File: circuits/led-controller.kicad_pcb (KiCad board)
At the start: 4 copper layers, 33.1 x 78.4 mm, 53 parts, among them J1 Conn_02x08_Odd_Even, Q1 Q_NPN_BEC, U1 ESP-WROOM-32, U2 IR-RX-TSOP34438, U3 SPH0645LM4H-B, U4 MCP73831T, U5 MAX98357AETE+T, U6 SI7020-A20, U7 PYQ2898, U7 housing-mounts, U8 TSL45315CL, U9 AP2112

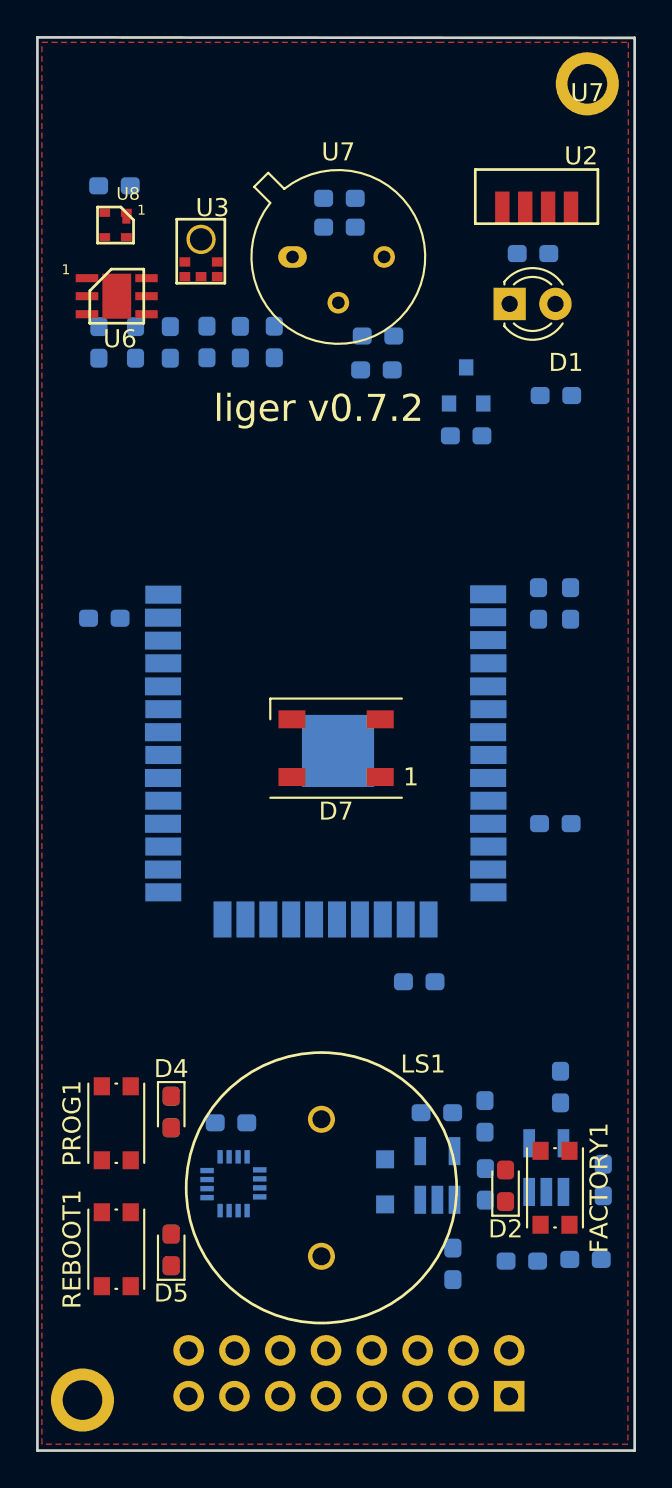
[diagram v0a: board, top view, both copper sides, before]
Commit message: sent to boardhouse
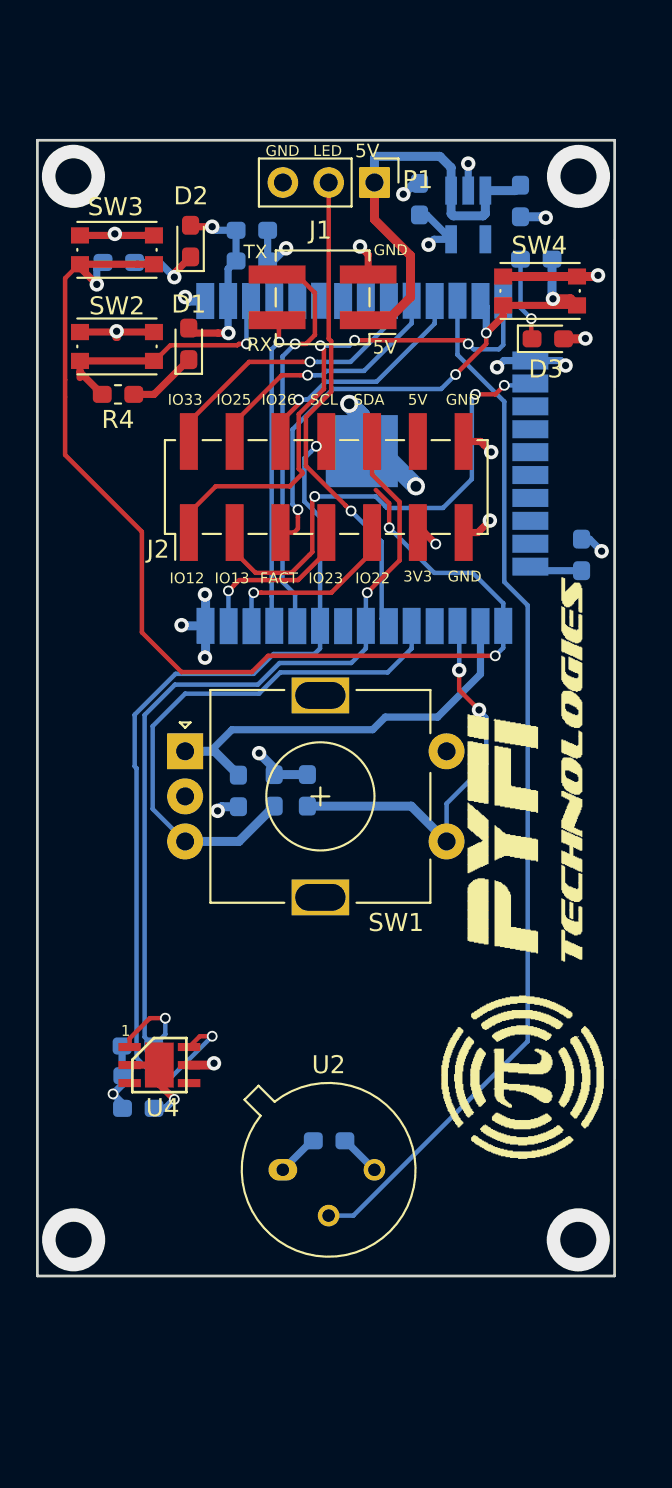
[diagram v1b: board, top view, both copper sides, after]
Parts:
- removed C10, C11: C_0.1uF, Capacitor_SMD:C_0603_1608Metric_Pad1.05x0.95mm_HandSolder
- removed C12, C7, C8, C9: C_1uF, Capacitor_SMD:C_0603_1608Metric_Pad1.05x0.95mm_HandSolder
- removed D4, D5: LED-0603-G, LED_SMD:LED_0603_1608Metric_Pad1.05x0.95mm_HandSolder
- removed D6: D_Schottky-BAT20JFILM, Diode_SMD:D_SOD-323_HandSoldering
- removed D7: WS2812B, LED_SMD:LED_WS2812B_PLCC4_5.0x5.0mm_P3.2mm
- removed FACTORY1, PROG1, REBOOT1: SW_PUSH, Button_Switch_SMD:SW_SPST_KMR2
- removed the LOGO at (157.2, 50.9)
- removed LS1: speaker-CVS-1508, open-automation:speaker-1508
- removed Q1: Q_NPN_BEC, Package_TO_SOT_SMD:SOT-23
- removed R10, R14, R15, R16: R_1k, Resistor_SMD:R_0603_1608Metric_Pad1.05x0.95mm_HandSolder
- removed R11: R_47.5, Resistor_SMD:R_0603_1608Metric_Pad1.05x0.95mm_HandSolder
- removed R19: R_2k, Resistor_SMD:R_0603_1608Metric_Pad1.05x0.95mm_HandSolder
- removed R20: R_100k, Resistor_SMD:R_0603_1608Metric_Pad1.05x0.95mm_HandSolder
- removed R22: R_10k, Resistor_SMD:R_0603_1608Metric_Pad1.05x0.95mm_HandSolder
- removed U5: MAX98357AETE+T, open-automation:MAX98357A
- removed U6: SI7020-A20, open-automation:SI7020-A20
- removed U7: PYQ2898, Package_TO_SOT_THT:TO-5-3
- removed U7: housing-mounts, open-automation:generic-housing-mounts-md
- removed U8: TSL45315CL, open-automation:LIGHT-SENSOR-TSL45315CL
- removed U9: AP2112, Package_TO_SOT_SMD:SOT-23-5_HandSoldering
- added J2: Conn_02x07_Odd_Even, Connector_PinHeader_2.54mm:PinHeader_2x07_P2.54mm_Vertical_SMD, F.Cu at (146.5, 74.2)
- added LOGO: , open-automation:LOGO, F.Cu at (158.8, 100.2)
- added P1: CONN_01X03, Connector_PinHeader_2.54mm:PinHeader_1x03_P2.54mm_Vertical, F.Cu at (149.2, 57.3)
- added SW1: Rotary_Encoder_Switch, Rotary_Encoder:RotaryEncoder_Alps_EC11E-Switch_Vertical_H20mm, F.Cu at (138.7, 88.8)
- added SW2: SW_PUSH, Button_Switch_SMD:SW_Push_1P1T_NO_CK_KMR2, F.Cu at (134.9, 66.4)
- added SW3: SW_PUSH, Button_Switch_SMD:SW_Push_1P1T_NO_CK_KMR2, F.Cu at (134.9, 61.0)
- added SW4: SW_PUSH, Button_Switch_SMD:SW_Push_1P1T_NO_CK_KMR2, F.Cu at (158.4, 63.3)
- C1: value C_10uF -> C_1uF
- C4: value C_100pF -> C_10uF
- C5: value C_0.1uF -> C_1uF
- D1: value LED -> LED_G; footprint LED_THT:LED_D3.0mm -> Diode_SMD:D_0603_1608Metric_Pad1.05x0.95mm_HandSolder
- D2: value LED-0603-G -> LED_G; footprint LED_SMD:LED_0603_1608Metric_Pad1.05x0.95mm_HandSolder -> Diode_SMD:D_0603_1608Metric_Pad1.05x0.95mm_HandSolder
- D3: value LED-0603-G -> LED_G; footprint LED_SMD:LED_0603_1608Metric_Pad1.05x0.95mm_HandSolder -> Diode_SMD:D_0603_1608Metric_Pad1.05x0.95mm_HandSolder; moved to F.Cu
- J1: value Conn_02x08_Odd_Even -> Conn_02x02_Odd_Even; footprint Connector_PinHeader_2.54mm:PinHeader_2x08_P2.54mm_Vertical -> Connector_PinHeader_2.54mm:PinHeader_2x02_P2.54mm_Vertical_SMD; moved to F.Cu
- R1, R7, R8: value R_47.5 -> R_10K
- R2, R6: value R_10k -> R_10K
- R3: value R_1k -> R_10K
- R4: value R_1k -> R_10K; moved to F.Cu
- R5: value 36 -> R_10K
- R9: value R_100k -> R_10K
- U1: value ESP-WROOM-32 -> AP2112; footprint open-automation:ESP-WROOM-32 -> Package_TO_SOT_SMD:SOT-23-5_HandSoldering
- U2: value IR-RX-TSOP34438 -> PIR-DIGITAL; footprint open-automation:TSOP75338TR -> Package_TO_SOT_THT:TO-5-3
- U3: value SPH0645LM4H-B -> ESP-WROOM-32; footprint open-automation:SPH0645LM4H-B -> open-automation:ESP-WROOM-32; moved to B.Cu
- U4: value MCP73831T -> SI7020-A20; footprint Package_TO_SOT_SMD:SOT-23-5_HandSoldering -> open-automation:SI7020-A20; moved to F.Cu
- moved J1 61.8 mm to (146.3, 63.6), turned to 180 degrees
- moved U2 55.5 mm to (144.1, 112.0)
- moved D2 55.2 mm to (139.0, 60.5)
- moved C3 52.3 mm to (146.7, 110.4)
- moved D3 51.1 mm to (158.8, 65.9)
- moved R8 41.6 mm to (136.1, 105.2), turned to 0 degrees
- moved R3 32.3 mm to (145.5, 91.0), turned to 90 degrees
- moved C2 27.2 mm to (142.4, 59.9), turned to 0 degrees
- moved R2 26.0 mm to (143.6, 91.0), turned to 90 degrees
- moved R7 25.4 mm to (136.1, 106.8)
- moved R5 25.3 mm to (135.0, 61.7), turned to 0 degrees
- moved R6 24.7 mm to (158.2, 61.5), turned to 180 degrees
- moved C1 22.3 mm to (157.3, 58.3), turned to 270 degrees
- moved U1 22.3 mm to (154.4, 59.1), turned to 270 degrees
- moved R9 22.3 mm to (160.7, 77.9), turned to 270 degrees
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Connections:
- C1 pad 1: /3V3 -> /5V
- C4 pad 1: Net-(C4-Pad1) -> /3V3
- C6 pad 1: /V_IN -> /3V3
- D1 pad 2: Net-(D1-Pad2) -> /3V3
- D3 pad 2: Net-(D3-Pad2) -> /3V3
- J1 pad 1: GND -> /5V
- J1 pad 2: GND -> /TXD
- J1 pad 4: /V_USB -> /RXD
- R1 pad 1: Net-(R1-Pad1) -> /CLK_IO
- R1 pad 2: /I2S_BCLK -> /3V3
- R2 pad 1: /3V3 -> /DT_IO
- R2 pad 2: /SCL -> /3V3
- R3 pad 1: /IR_RX -> /SW_IO
- R3 pad 2: Net-(R3-Pad2) -> /3V3
- R4 pad 1: Net-(Q1-Pad1) -> /microcontroller/EN
- R4 pad 2: /IR_TX -> Net-(D1-Pad1)
- R5 pad 1: /3V3 -> /microcontroller/PROG
- R5 pad 2: Net-(D1-Pad2) -> Net-(D2-Pad1)
- R6 pad 1: /3V3 -> /microcontroller/FACT
- R6 pad 2: /SDA -> Net-(D3-Pad1)
- R7 pad 1: /I2S_WS -> /3V3
- R7 pad 2: Net-(R7-Pad2) -> /microcontroller/SCL
- R8 pad 1: /PIR -> /3V3
- R8 pad 2: Net-(C4-Pad1) -> /microcontroller/SDA
- R9 pad 2: Net-(R11-Pad2) -> Net-(R9-Pad2)
- U1 pad 1: GND -> /5V
- U1 pad 2: /3V3 -> GND
- U1 pad 3: /EN -> /5V
- U1 pad 4: Net-(U1-Pad4) -> (no net)
- U1 pad 5: Net-(U1-Pad5) -> /3V3
- U3 pad 1: /I2S_WS -> GND
- U3 pad 2: GND -> /3V3
- U3 pad 3: GND -> /microcontroller/EN
- U3 pad 4: /I2S_BCLK -> Net-(U3-Pad4)
- U3 pad 5: /3V3 -> Net-(U3-Pad5)
- U3 pad 6: Net-(R11-Pad2) -> /microcontroller/IO34
- U4 pad 1: Net-(D3-Pad1) -> /microcontroller/SDA
- U4 pad 3: /V_BAT -> (no net)
- U4 pad 4: /V_USB -> (no net)
- U4 pad 5: Net-(R19-Pad2) -> /3V3
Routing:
- net /microcontroller/PROG: track 0.00 -> 64.0 mm, vias 0 -> 3
- net /PIR_IO: track 0.00 -> 57.7 mm
- net GND: track 0.00 -> 51.7 mm, vias 0 -> 22
- net /microcontroller/SCL: track 0.00 -> 50.5 mm, vias 0 -> 2
- net /microcontroller/SDA: track 0.00 -> 50.0 mm, vias 0 -> 2
- net /microcontroller/FACT: track 0.00 -> 31.6 mm, vias 0 -> 4
- net /DT_IO: track 0.00 -> 30.3 mm
- net /3V3: track 0.00 -> 29.2 mm, vias 0 -> 9
- net /microcontroller/IO12: track 0.00 -> 29.1 mm, vias 0 -> 3
- net /microcontroller/IO13: track 0.00 -> 27.2 mm, vias 0 -> 3
- net /LED_IO: track 0.00 -> 27.2 mm, vias 0 -> 1
- net /CLK_IO: track 0.00 -> 24.3 mm
- net /5V: track 0.00 -> 23.9 mm
- net /RXD: track 0.00 -> 22.4 mm, vias 0 -> 1
- net /SW_IO: track 0.00 -> 22.1 mm, vias 0 -> 2
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- added copper zone on In2.Cu, net /3V3
- added copper zone on In1.Cu, net GND
- removed copper zone on F.Cu, net GND
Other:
- board size 33.1 x 78.4 mm -> 32 x 63 mm
- board text added: "FACT"
- board text added: "IO12"
- board text added: "IO13"
- board text added: "IO22"
- board text added: "IO23"
- board text added: "IO25"
- board text added: "IO26"
- board text added: "IO33"
- board text added: "LED"
- board text added: "SCL"
- board text added: "SDA"
- board text removed: "BAT+"
- board text removed: "BCLK"
- board text removed: "PROG"
- board text removed: "T1"
- board text removed: "T2"
- board text removed: "T3"
- board text removed: "T4"
- board text removed: "WS"
- board text removed: "ZD"
- board text removed: "liger v0.7.2"
